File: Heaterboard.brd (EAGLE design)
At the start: 132.1 x 30.1 mm, 15 parts, among them IC1 EK-TM4C123GXLP, J1 POWER_JACK, U1 CSD18504KCS, U2 LM35DT, U3 TLC5926IDBQRDBQ24-M

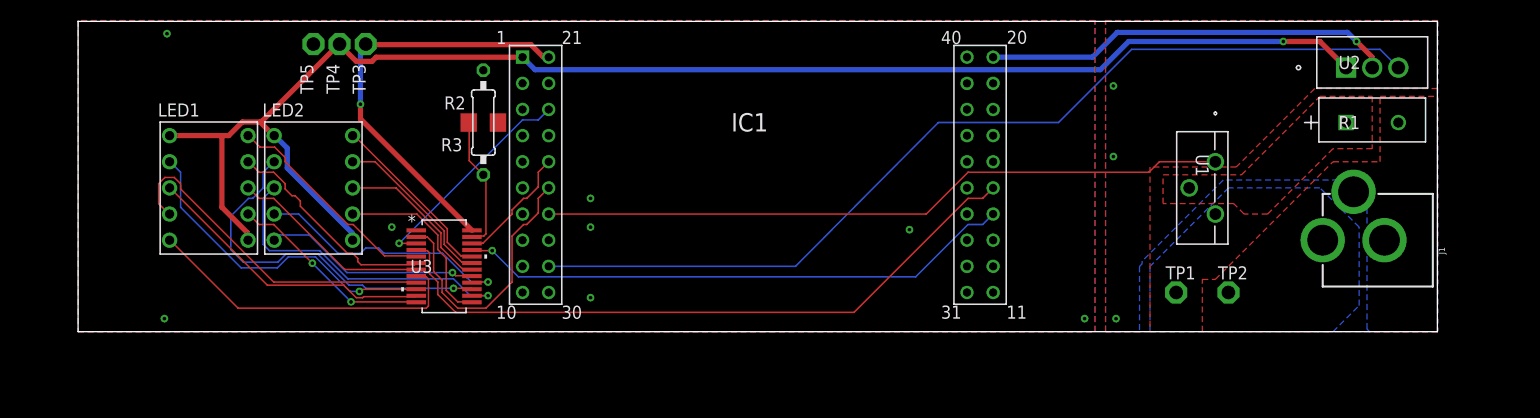
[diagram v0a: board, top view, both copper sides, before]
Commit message: final checkpoint
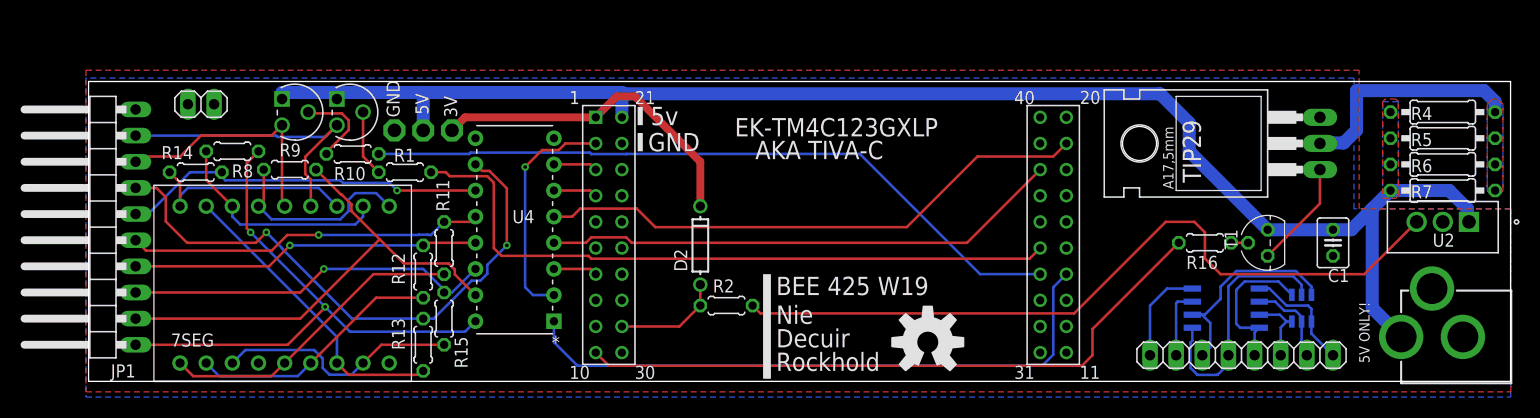
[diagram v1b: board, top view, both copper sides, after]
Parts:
- removed IC1: EK-TM4C123GXLP, EK-TM4C123GXL:TM4C123LAUNCHPAD
- removed LED1, LED2: LA-401AD, led-7-segment:LA-401
- removed R3: (no value), resistor:0207/10
- removed TP1, TP2, TP3, TP4, TP5: PTR1PAD1-13, testpad:P1-13
- added 3V, 5V, GND: PTR1PAD1-13, testpad:P1-13
- added 7SEG: NTE3074, partlibrary:NTE3074
- added C1: 10uF, resistor:C025-030X050
- added D2: (no value), adafruit:DO-1N4148
- added IC2: ATTINY10, adafruit:SOT23-6
- added JP1: (no value), pinhead:1X10/90
- added JP2: (no value), pinhead:1X02
- added JP4: (no value), pinhead:1X08
- added LOGO1: OSHW-LOGOL, SparkFun-Aesthetics:OSHW-LOGO-L
- added R10, R16: 330, resistor:0204/5
- added R11, R12, R13, R14, R15, R8, R9: 150, resistor:0204/5
- added R4, R5, R6, R7: 200, resistor:0207/10
- added T1: 2N3904, transistor:TO92
- added TIP29: TIP29AG, partlibrary:TO220
- added TIVA: EK-TM4C123GXLP, EK-TM4C123GXL:TM4C123LAUNCHPAD
- added U4: ULN2003A, partlibrary:DIP-16
- added U5: W25Q32FV, SparkFun-IC-Memory:SOIC-8
- R1: value PWR220T-20-50R0F -> 330; device partlibrary:BO_PWR220T -> resistor:0204/5
- R2: value (none) -> 10k; device resistor:R1206 -> resistor:0204/5
- U1: value CSD18504KCS -> 2N3906; device partlibrary:KCS3 -> partlibrary:TO-92_2
- U3: value TLC5926IDBQRDBQ24-M -> 2N3906; device partlibrary:DBQ24-M -> partlibrary:TO-92_2
- moved R1 96.6 mm to (31.8, 21.8), turned to 180 degrees
- moved U1 86.0 mm to (22.4, 26.4)
- moved R2 29.6 mm to (63.0, 8.89), turned to 180 degrees
- moved U2 17.1 mm to (130.0, 16.0), turned to 180 degrees
- moved U3 15.8 mm to (27.7, 26.4), turned to 270 degrees
- moved J1 12.1 mm to (142.2, 5.84)
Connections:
- removed net HEATER_ON: R1.1, U1.2
- removed net LE: IC1.15, U3.4
- removed net N$11: LED1.3, U3.11
- removed net N$18: LED2.8, U3.18
- removed net N$40: R2.1, R3.1, U3.23
- removed net N$6: LED1.9, U3.6
- removed net N$7: LED1.8, U3.7
- removed net OE: IC1.14, U3.21
- removed net PWR_ON: IC1.27, U1.1
- removed net SDI: IC1.26, U3.2
- removed net SDO: IC1.25, U3.22
- removed net VDD: J1.PWR, TP1.TP, U1.3
- removed net VSS: J1.GND, J1.GNDBREAK, R1.2, TP2.TP
- new net 1C: JP1.1, R8.2, U4.16
- new net 2C: JP1.2, R9.2, U4.15
- new net 3C: JP1.3, R15.2, U4.14
- new net 4C: JP1.4, R12.2, U4.13
- new net 5C: JP1.5, R11.2, U4.12
- new net 6C: JP1.6, R14.2, U4.11
- new net 7C: JP1.7, R13.2, U4.10
- new net ANODE1: 7SEG.14, JP1.8, U1.1
- new net ANODE2: 7SEG.13, JP1.9, U3.1
- new net HEATER_COM: R4.1, R5.1, R6.1, R7.1, TIP29.2
- new net N$1: R2.1, U2.3
- new net N$21: IC2.3, JP4.3, U5.3
- new net N$23: IC2.5, JP4.5, U5.5
- new net N$24: IC2.6, JP4.6, U5.6
- new net N$25: JP4.7, U5.7
- new net N$26: JP4.8, U5.8
- new net N$3: R16.1, T1.2
- new net N$4: T1.3, TIP29.1
- new net PA2: TIVA.11
- new net PA3: TIVA.12
- new net PA4: TIVA.13
- new net PA5: TIVA.8
- new net PA6: TIVA.9
- new net PB0: TIVA.3, U4.7
- new net PB1: TIVA.4, U4.6
- new net PB2: TIVA.19, U4.5
- new net PB3: TIVA.38, U4.4
- new net PB4: TIVA.7, U4.3
- new net PB5: TIVA.2, U4.2
- new net PB6: TIVA.14, U4.1
- new net PB7: TIVA.15
- new net PC4: TIVA.37
- new net PC5: TIVA.36
- new net PC6: R1.1, TIVA.35
- new net PC7: R10.1, TIVA.34
- new net PD1: TIVA.24
- new net PD2: TIVA.25
- new net PD3: TIVA.26
- new net PD6: TIVA.33
- new net PD7: TIVA.32
- new net PE0: TIVA.18
- new net PE1: TIVA.27
- new net PE2: TIVA.28
- new net PE4: TIVA.5
- new net PE5: TIVA.6
- new net PF0: TIVA.17
- new net PF1: TIVA.30
- new net PF2: TIVA.40
- new net PF3: TIVA.39
- new net PF4: TIVA.31
- new net P_ON: R16.2, TIVA.10
- new net RESET: TIVA.16
- net +3V3: now also 3V.TP, D2.C, TIVA.1; no longer IC1.1, LED1.1, LED1.6, LED2.1, LED2.6, TP4.TP, U2.1
- net +5V: now also 5V.TP, C1.1, J1.PWR, R4.2, R5.2, R6.2, R7.2, T1.1, TIVA.21, U1.3, U2.1, U3.3; no longer IC1.21, TP3.TP, U3.24
- net CLK: now also TIVA.23; no longer IC1.23, U3.3
- net GND: now also C1.2, GND.TP, J1.GND, J1.GNDBREAK, JP1.10, JP2.1, JP2.2, TIP29.3, TIVA.20, TIVA.22, U4.8; no longer IC1.20, IC1.22, R2.2, R3.2, TP5.TP, U3.1
- net N$10: now also IC2.4, JP4.4, U5.4; no longer LED1.2, U3.10
- net N$12: now also 7SEG.10, 7SEG.15, R9.1; no longer LED1.7, U3.12
- net N$13: now also 7SEG.3, 7SEG.8, R15.1; no longer LED2.7, U3.13
- net N$14: now also 7SEG.2, 7SEG.6, R12.1; no longer LED2.3, U3.14
- net N$15: now also 7SEG.1, 7SEG.5, R11.1; no longer LED2.2, U3.15
- net N$16: now also 7SEG.12, 7SEG.18, R14.1; no longer LED2.4, U3.16
- net N$17: now also 7SEG.17, 7SEG.7, R13.1; no longer LED2.5, U3.17
- net N$19: now also IC2.1, JP4.1, U5.1; no longer LED2.9, U3.19
- net N$20: now also IC2.2, JP4.2, U5.2; no longer LED2.10, U3.20
- net N$5: now also R10.2, U1.2; no longer LED1.10, U3.5
- net N$8: now also R1.2, U3.2; no longer LED1.5, U3.8
- net N$9: now also 7SEG.11, 7SEG.16, R8.1; no longer LED1.4, U3.9
- net T-SENSE: now also D2.A, R2.2, TIVA.29; no longer IC1.29, U2.3
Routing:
- net +3V3: track 148.1 -> 32.4 mm, vias 1 -> 0
- net +5V: track 41.1 -> 146.9 mm, vias 1 -> 0
- net T-SENSE: track 92.0 -> 10.5 mm
- net N$1: track 0.00 -> 74.2 mm
- net PC7: track 0.00 -> 69.2 mm
- net PWR_ON: track 66.9 -> 0.00 mm
- net PC6: track 0.00 -> 66.8 mm
- net LE: track 65.5 -> 0.00 mm
- net P_ON: track 0.00 -> 63.6 mm
- net PB6: track 0.00 -> 60.3 mm
- net 7C: track 0.00 -> 56.6 mm, vias 0 -> 2
- net 1C: track 0.00 -> 54.7 mm, vias 0 -> 2
- net OE: track 54.2 -> 0.00 mm, vias 1 -> 0
- net PB2: track 0.00 -> 54.2 mm
- net PB3: track 0.00 -> 50.6 mm
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- added copper zone on layer 1, net +5V
- added copper zone on layer 16, net +5V
- added copper zone on layer 1, net HEATER_COM
- added copper zone on layer 16, net HEATER_COM
- removed copper zone on layer 1, net DISCONNECT
- removed copper zone on layer 16, net DISCONNECT
- removed copper zone on layer 1, net HEATER_ON
- removed copper zone on layer 16, net VDD
- removed copper zone on layer 1, net VSS
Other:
- board size 132.1 x 30.1 mm -> 138.2 x 29.1 mm
- board text added: "1C"
- board text added: "2C"
- board text added: "3C"
- board text added: "4C"
- board text added: "5C"
- board text added: "5V ONLY!"
- board text added: "5v"
- board text added: "6C"
- board text added: "7C"
- board text added: "AKA TIVA-C"
- board text added: "An1"
- board text added: "An2"
- board text added: "BEE 425 W19"
- board text added: "Decuir"
- board text added: "GND"
- board text added: "Nie"
- board text added: "PB0 > 7B, 7C > G1,G2 PB1 > 6B, 6C > F1,F2 PB2 > 5B, 5C > E1,E2 PB3 > 4B, 4C > D1,D2 PB4 > 3B, 3C > C1,C2 PB5 > 2B, 2C > B1,B2 PB6 > 1B, 1C > A1,A2 PC6 > ANODE2 PC6 > ANODE1 PE3 > Sensor PA7 > Heater"
- board text added: "Rockhold"
- board text added: "Secrets!"
